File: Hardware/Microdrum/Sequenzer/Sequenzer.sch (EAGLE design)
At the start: 20 parts

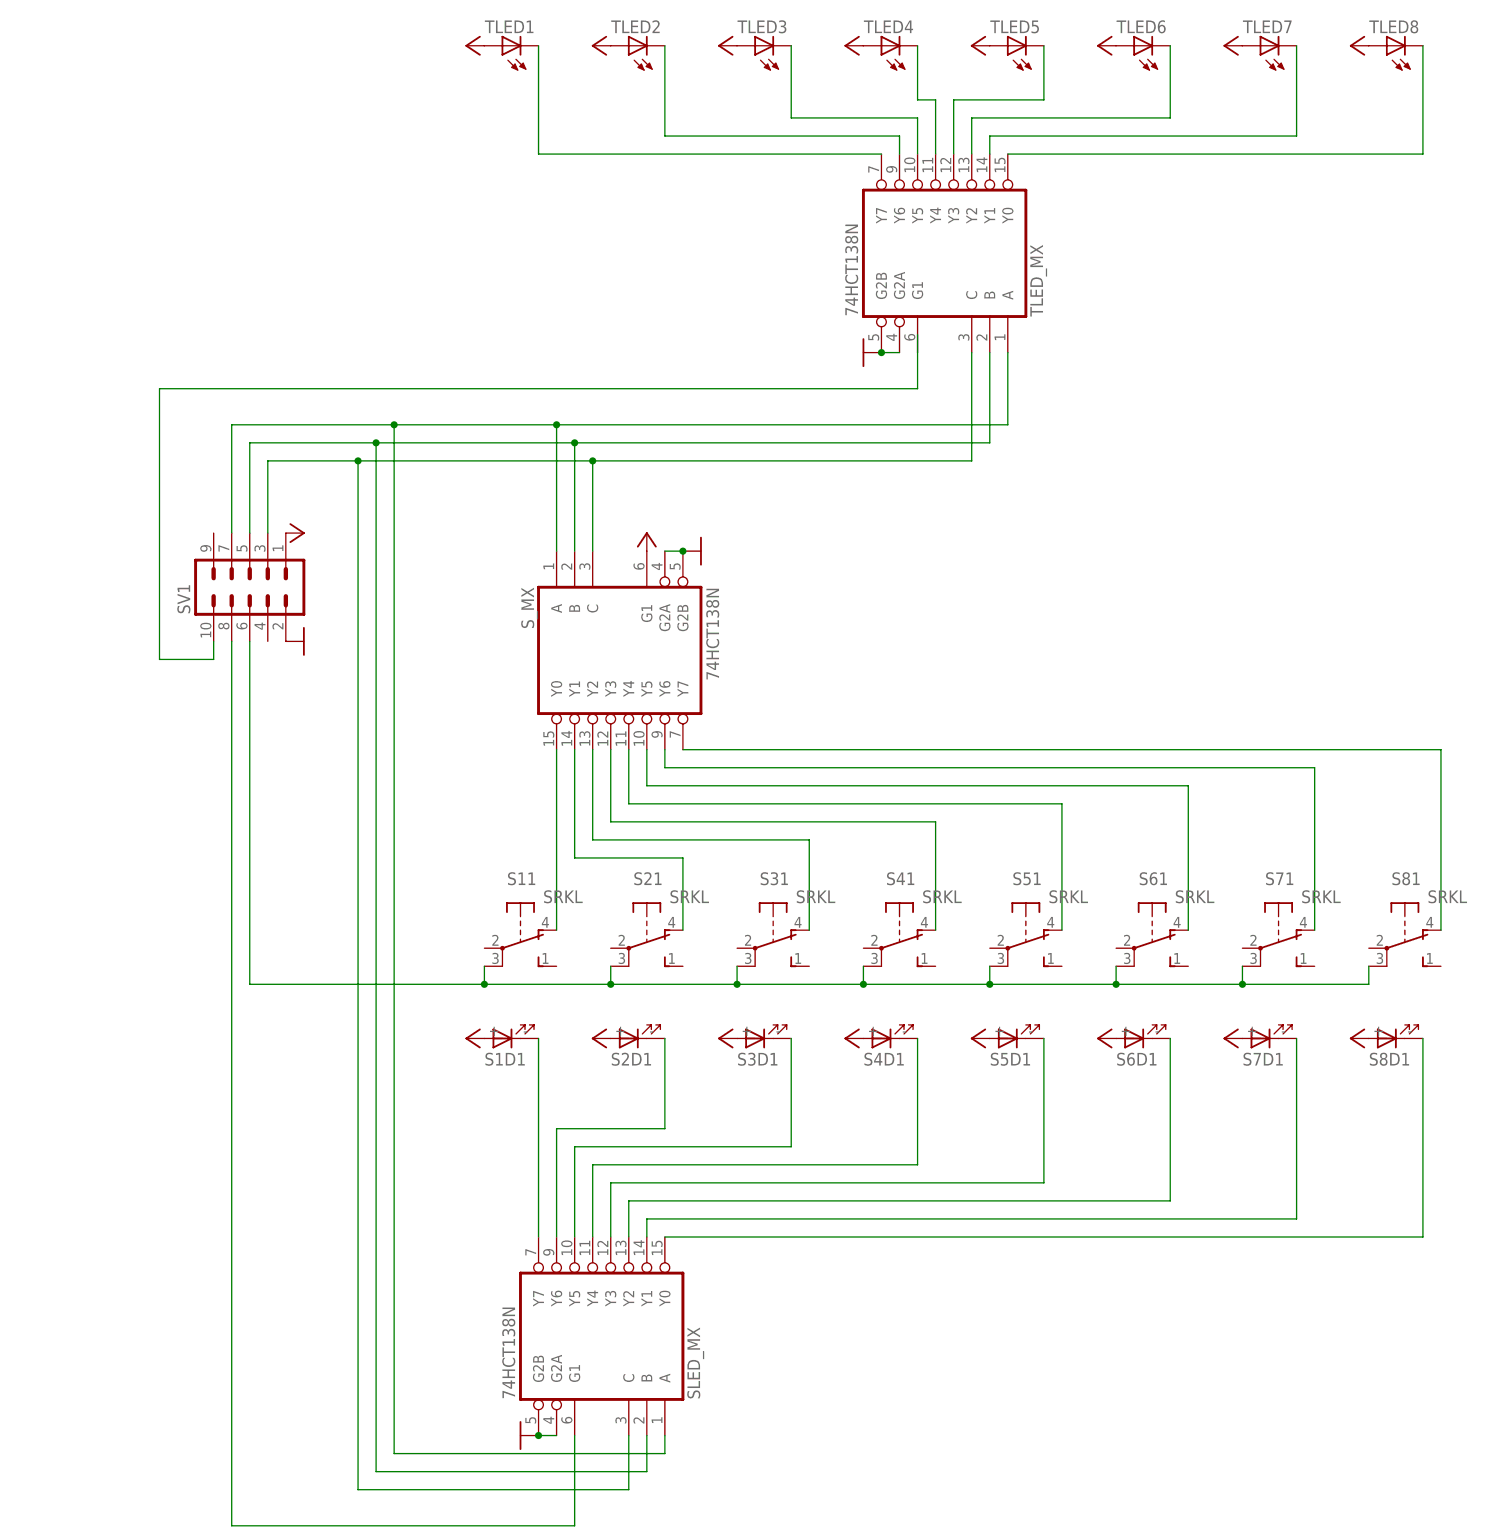
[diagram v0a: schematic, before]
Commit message: Langsam nimmt es Form an
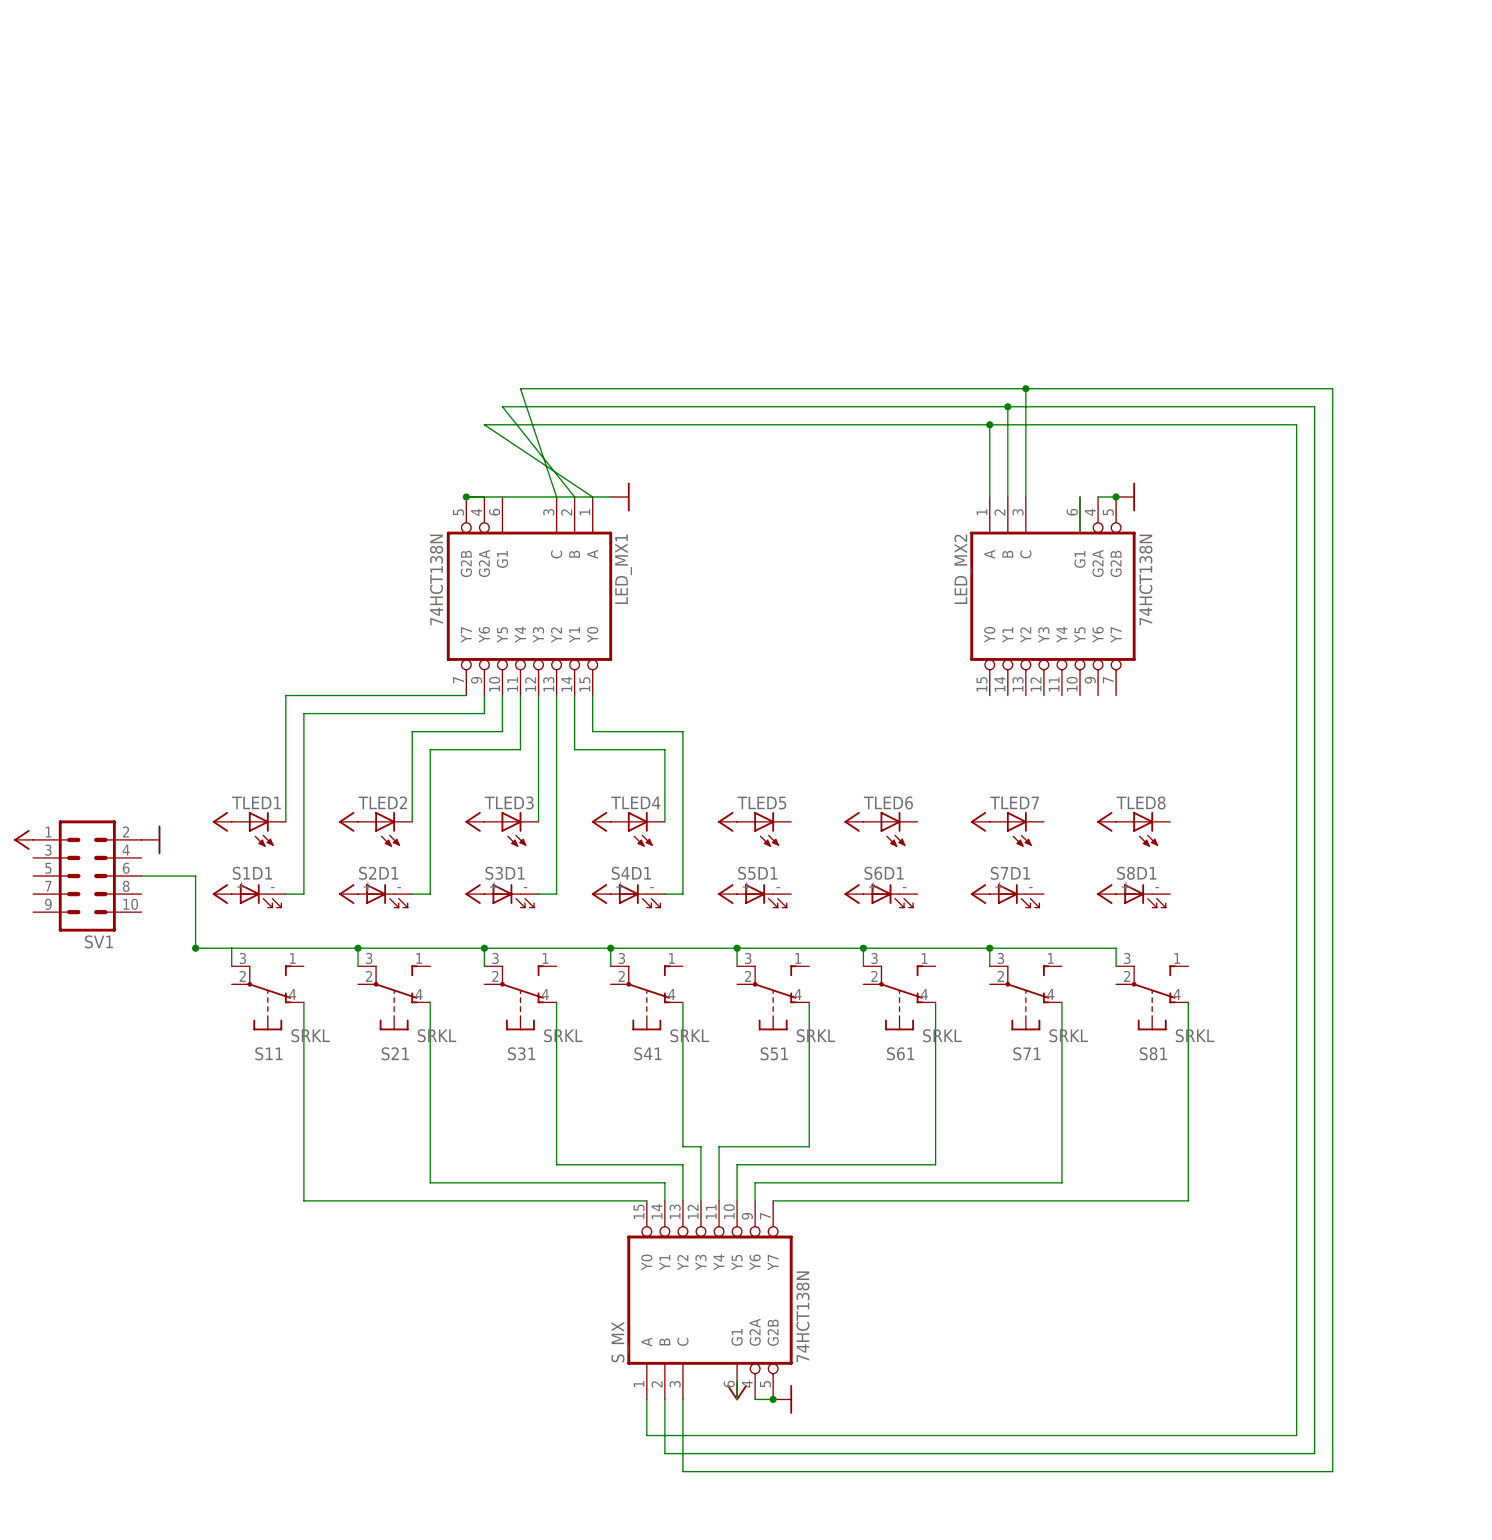
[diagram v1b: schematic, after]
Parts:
- removed SLED_MX, TLED_MX: 74HCT138N, 74xx-eu:74HCT138N
- added LED_MX1, LED_MX2: 74HCT138N, 74xx-eu:74HCT138N
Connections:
- net S1 renamed N$11
- net S2 renamed N$10
- net S3 renamed N$9
- net S4 renamed N$8
- net S5 renamed N$7
- net S6 renamed N$6
- net S7 renamed N$5
- net S8 renamed N$4
- removed net 1: SLED_MXA.A, SV1.7, S_MXA.A, TLED_MXA.A
- removed net 2: SLED_MXA.B, SV1.5, S_MXA.B, TLED_MXA.B
- removed net 3: SLED_MXA.C, SV1.3, S_MXA.C, TLED_MXA.C
- removed net SLED1: S1D1.C, SLED_MXA.Y7
- removed net SLED2: S2D1.C, SLED_MXA.Y6
- removed net SLED3: S3D1.C, SLED_MXA.Y5
- removed net SLED4: S4D1.C, SLED_MXA.Y4
- removed net SLED5: S5D1.C, SLED_MXA.Y3
- removed net SLED6: S6D1.C, SLED_MXA.Y2
- removed net SLED7: S7D1.C, SLED_MXA.Y1
- removed net SLED8: S8D1.C, SLED_MXA.Y0
- removed net SLED_EN: SLED_MXA.G1, SV1.8
- removed net TLED1: TLED1.C, TLED_MXA.Y7
- removed net TLED2: TLED2.C, TLED_MXA.Y6
- removed net TLED3: TLED3.C, TLED_MXA.Y5
- removed net TLED4: TLED4.C, TLED_MXA.Y4
- removed net TLED5: TLED5.C, TLED_MXA.Y3
- removed net TLED6: TLED6.C, TLED_MXA.Y2
- removed net TLED7: TLED7.C, TLED_MXA.Y1
- removed net TLED8: TLED8.C, TLED_MXA.Y0
- new net N$1: LED_MX1A.A, LED_MX2A.A, S_MXA.A
- new net N$12: LED_MX1A.Y7, TLED1.C
- new net N$13: LED_MX1A.Y6, S1D1.C
- new net N$14: LED_MX1A.Y5, TLED2.C
- new net N$15: LED_MX1A.Y4, S2D1.C
- new net N$16: LED_MX1A.Y3, TLED3.C
- new net N$17: LED_MX1A.Y2, S3D1.C
- new net N$18: LED_MX1A.Y1, TLED4.C
- new net N$19: LED_MX1A.Y0, S4D1.C
- new net N$2: LED_MX1A.B, LED_MX2A.B, S_MXA.B
- new net N$3: LED_MX1A.C, LED_MX2A.C, S_MXA.C
- net GND: now also LED_MX1A.G2A, LED_MX1A.G2B, LED_MX2A.G2A, LED_MX2A.G2B; no longer SLED_MXA.G2A, SLED_MXA.G2B, TLED_MXA.G2A, TLED_MXA.G2B
- net TLED_EN: now also LED_MX2A.G1; no longer SV1.10, TLED_MXA.G1
- net VCC: now also SV1.1
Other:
- moved on the sheet: S11, S1D1, S21, S2D1, S31, S3D1, S41, S4D1, S51, S5D1, S61, S6D1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
